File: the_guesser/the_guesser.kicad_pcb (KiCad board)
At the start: 4 copper layers, 24 x 72 mm, 58 parts, among them J1 USB_B_Mini, J3 BMI-S-209-F, U2 ESP32-S3, U3 W25Q128JVS, U5 CC1101RGPR, U6 CC1190RGVR, U7 B39921B3728U410, X1 STDCRG2-27M, X2 ECS-3953M-400-AU-TR

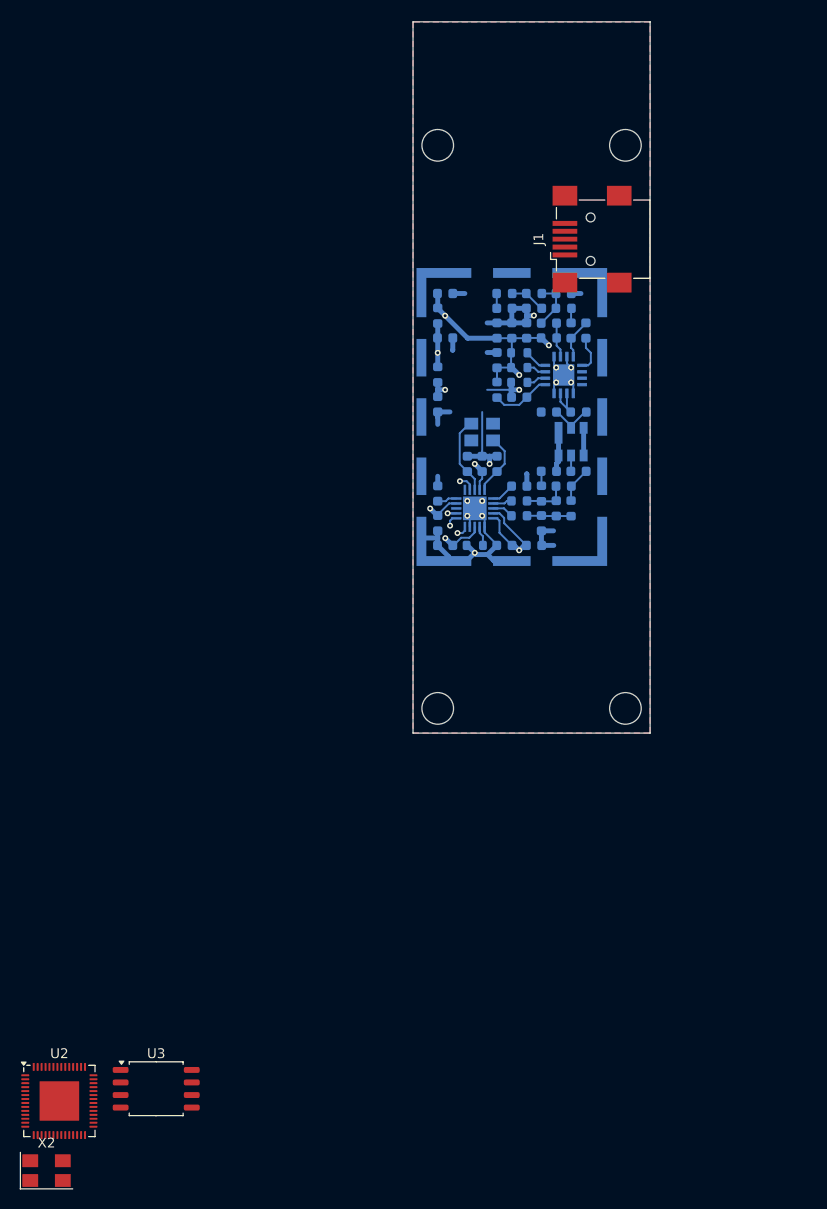
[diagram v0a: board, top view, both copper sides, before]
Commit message: Started Guesser sensor selection
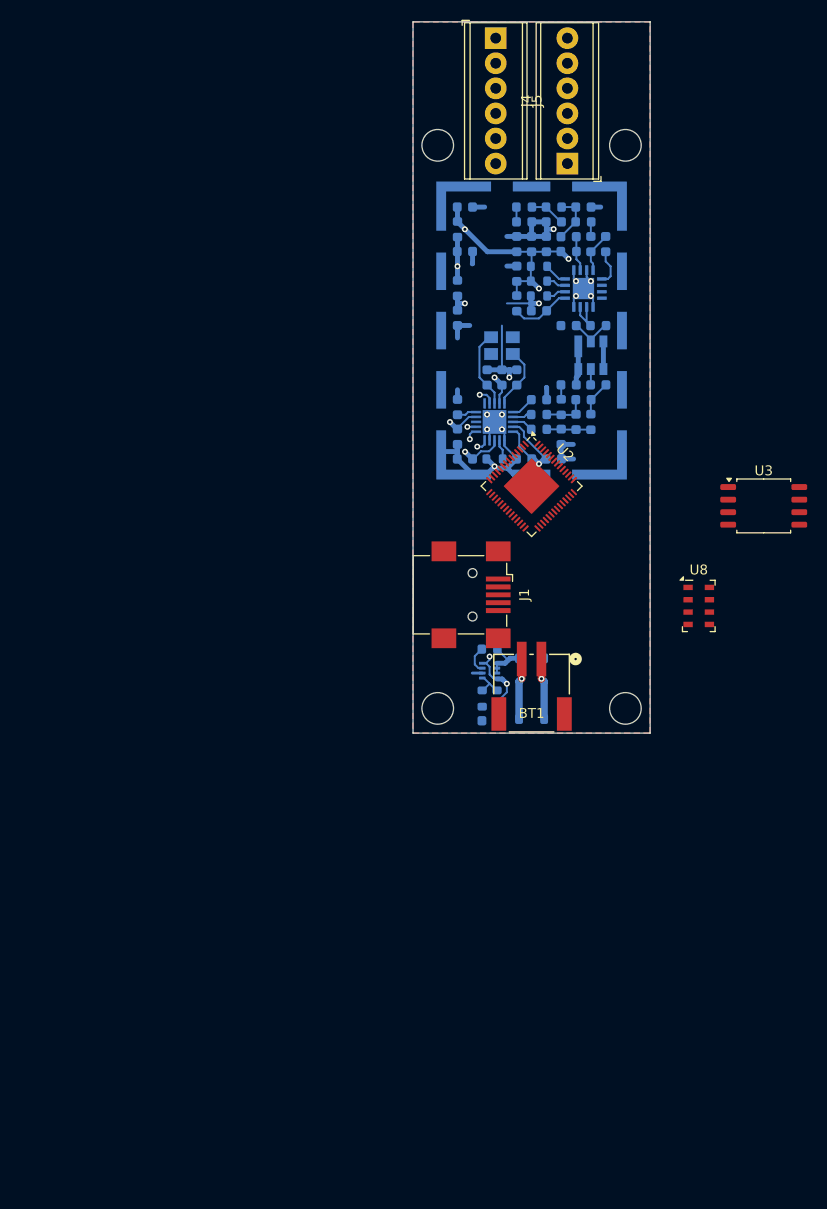
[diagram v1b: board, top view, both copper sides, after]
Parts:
- removed X2: ECS-3953M-400-AU-TR, Crystal:Crystal_SMD_5032-4Pin_5.0x3.2mm
- added BT1: Battery_Cell, locals_but_working_PLEASE:CONN2_1775469-2_TEC, F.Cu at (212.0, 100.0)
- added C4: 10u, Capacitor_SMD:C_0603_1608Metric, B.Cu at (207.8, 98.8)
- added D1: MB6S, Package_TO_SOT_SMD:TO-269AA, B.Cu at (212.0, 95.5)
- added J4: Screw_Terminal_01x06, TerminalBlock_Phoenix:TerminalBlock_Phoenix_MPT-0,5-6-2.54_1x06_P2.54mm_Horizontal, F.Cu at (215.6, 42.4)
- added J5: Screw_Terminal_01x06, TerminalBlock_Phoenix:TerminalBlock_Phoenix_MPT-0,5-6-2.54_1x06_P2.54mm_Horizontal, F.Cu at (208.4, 29.6)
- added L3: 0.47u, Inductor_SMD:L_0603_1608Metric, B.Cu at (207.8, 91.5)
- added R2: 5.36k, Resistor_SMD:R_0603_1608Metric, B.Cu at (208.5, 96.5)
- added R3: 1.2k, Resistor_SMD:R_0603_1608Metric, B.Cu at (207.0, 96.5)
- added U10: TPS61033DRLR, Package_TO_SOT_SMD:SOT-583-8, B.Cu at (207.8, 93.7)
- added U8: MS5607-02BA, Package_LGA:LGA-8_3x5mm_P1.25mm, F.Cu at (228.9, 87.1)
- moved U3 85.2 mm to (235.5, 77.0)
- moved U2 78.5 mm to (212.0, 75.0), turned to -45 degrees
- moved J1 37.9 mm to (206.0, 86.0), turned to -90 degrees
- moved C1 8.98 mm to (204.5, 58.0)
- moved X1 8.98 mm to (209.0, 60.8)
- moved C101 8.98 mm to (210.5, 64.0)
- moved C111 8.98 mm to (212.8, 66.2)
- moved C121 8.98 mm to (216.5, 68.5)
- moved C122 8.98 mm to (217.2, 66.2)
- moved C123 8.98 mm to (218.8, 64.8)
- moved C124 8.98 mm to (215.8, 64.8)
- moved C125 8.98 mm to (215.8, 58.8)
- moved C131 8.98 mm to (215.0, 70.0)
- moved C132 8.98 mm to (212.8, 57.2)
- moved C141 8.98 mm to (214.2, 72.2)
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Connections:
- net V_{BAT} renamed V_{USB}
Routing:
- net VCC: track 4.34 -> 13.1 mm, vias 1 -> 3
- net /BT-: track 0.00 -> 6.19 mm, vias 0 -> 1
- net /BT+: track 0.00 -> 6.19 mm, vias 0 -> 1
- net V_{B}: track 0.00 -> 5.02 mm
- net Net-(U10-FB): track 0.00 -> 3.04 mm
- net Net-(U10-SW): track 0.00 -> 2.76 mm
- net GND: track 62.5 -> 63.5 mm
